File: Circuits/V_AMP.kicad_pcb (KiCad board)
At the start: 2 copper layers, 103 x 153.5 mm, 138 parts, among them P1 INPUT, P2 GAIN_ADJ, P3 OUTPUT (0-5V), P4 POWER, U1 wOPA177, U2 LM393, U3 OPA177

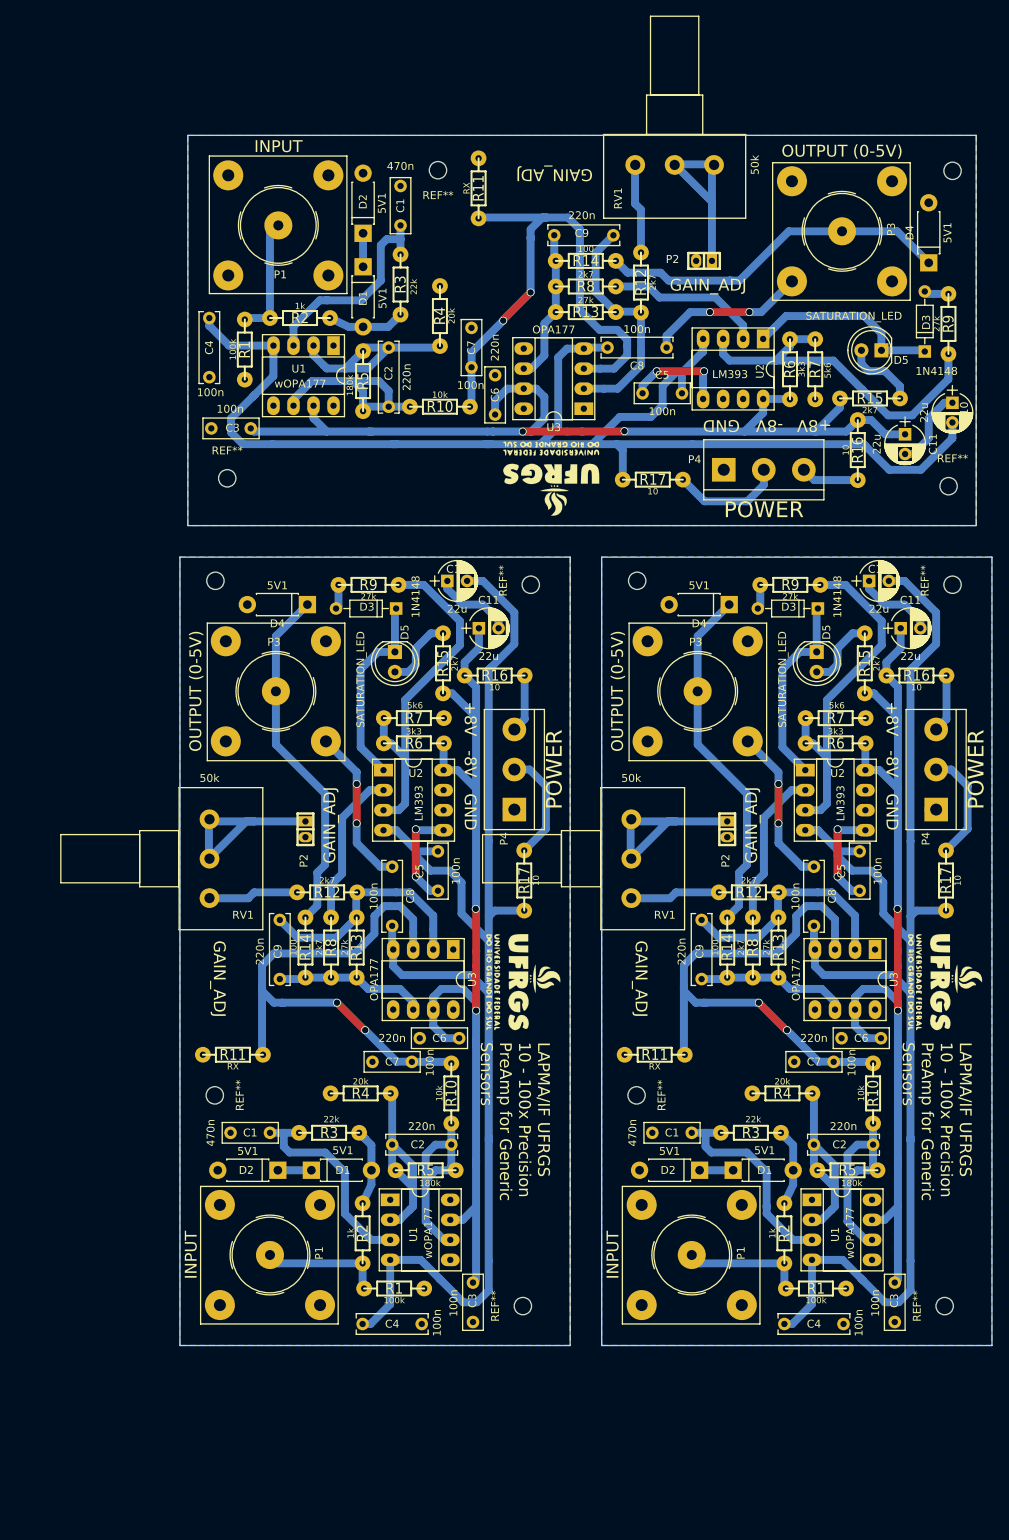
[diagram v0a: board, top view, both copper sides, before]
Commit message: EDIT: Page SETUP
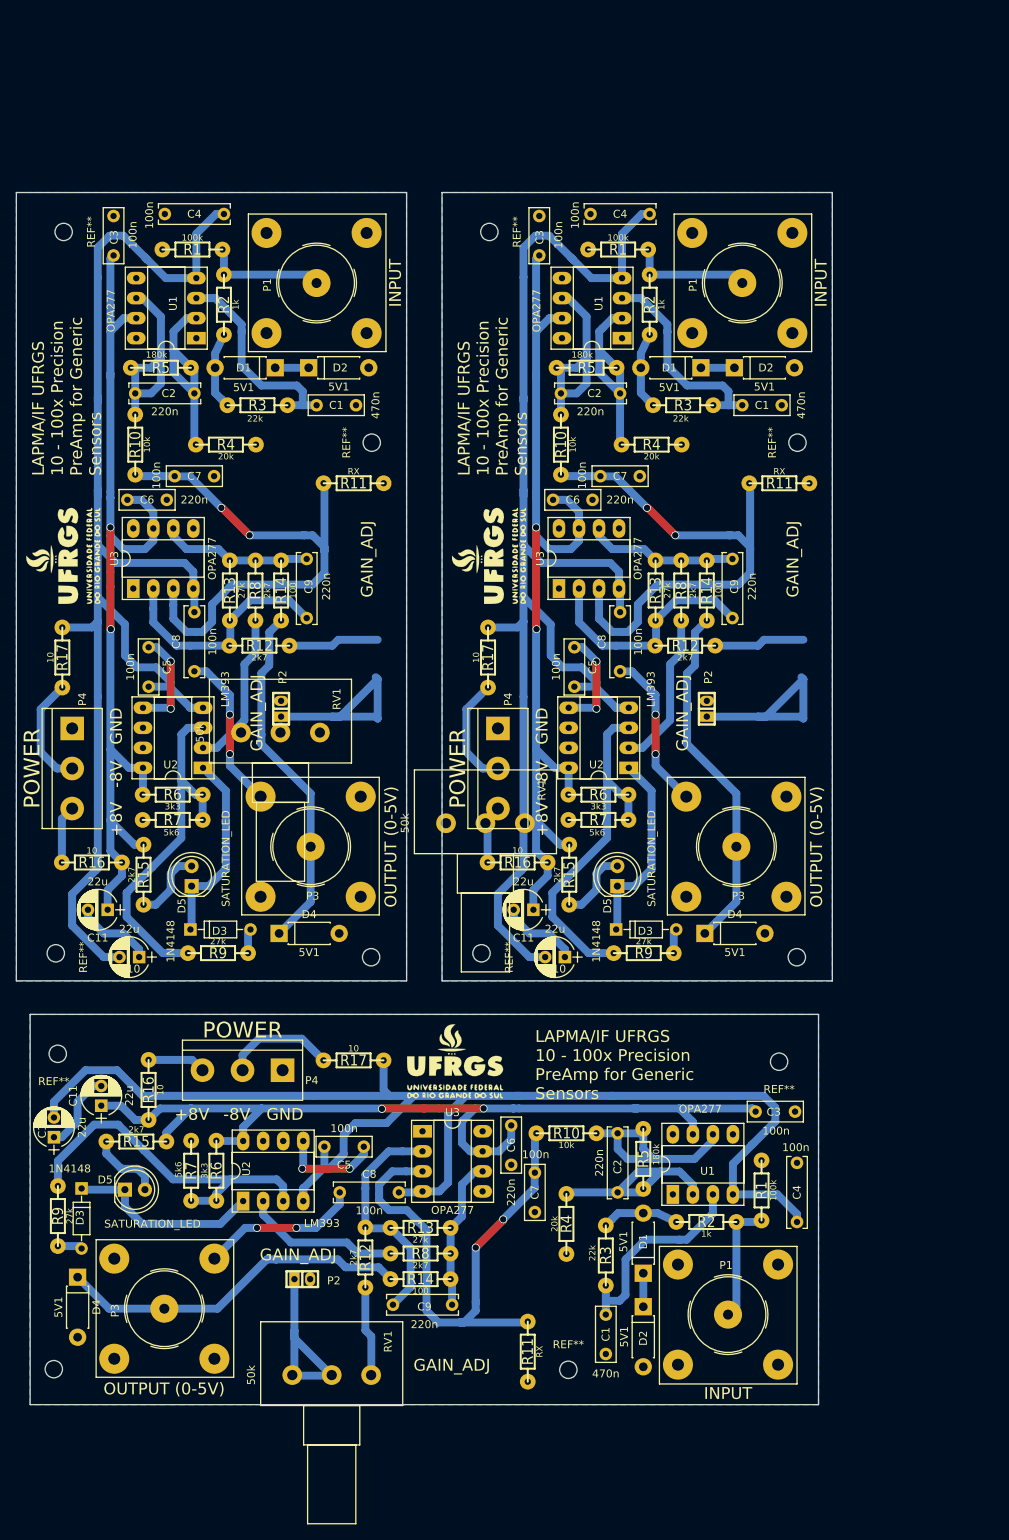
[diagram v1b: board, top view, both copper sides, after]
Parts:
- removed the C1 at (135.9, 152.0)
- removed the C1 at (82.4, 152.0)
- removed the C10 at (158.4, 82.0)
- removed the C10 at (104.9, 82.0)
- removed the C11 at (162.4, 88.0)
- removed the C11 at (108.9, 88.0)
- removed the C2 at (158.9, 153.5)
- removed the C2 at (105.4, 153.5)
- removed the C3 at (161.7, 176.0)
- removed the C3 at (108.2, 176.0)
- removed the C4 at (155.2, 176.3)
- removed the C4 at (101.7, 176.3)
- removed the C5 at (157.2, 121.3)
- removed the C5 at (103.7, 121.3)
- removed the C6 at (154.9, 140.0)
- removed the C6 at (101.4, 140.0)
- removed the C7 at (148.9, 143.0)
- removed the C7 at (95.4, 143.0)
- removed the C8 at (151.4, 118.3)
- removed the C8 at (97.9, 118.3)
- removed the C9 at (137.2, 125.0)
- removed the C9 at (83.7, 125.0)
- removed the D1 at (141.2, 156.8)
- removed the D1 at (87.7, 156.8)
- removed the D2 at (136.9, 156.8)
- removed the D2 at (83.4, 156.8)
- removed the D3 at (151.9, 85.5)
- removed the D3 at (98.4, 85.5)
- removed the D4 at (140.7, 85.0)
- removed the D4 at (87.2, 85.0)
- removed the D5 at (151.8, 91.0)
- removed the D5 at (98.3, 91.0)
- removed the G*** at (168.0, 133.0)
- removed the G*** at (114.5, 133.0)
- removed the P1 at (135.9, 167.5)
- removed the P1 at (82.4, 167.5)
- removed the P2 at (140.4, 113.5)
- removed the P2 at (86.9, 113.5)
- removed the P3 at (136.7, 96.0)
- removed the P3 at (83.2, 96.0)
- removed the P4 at (166.9, 111.0)
- removed the P4 at (113.4, 111.0)
- removed the R1 at (151.7, 171.8)
- removed the R1 at (98.2, 171.8)
- removed the R10 at (158.9, 147.0)
- removed the R10 at (105.4, 147.0)
- removed the R11 at (131.2, 142.1)
- removed the R11 at (77.7, 142.1)
- removed the R12 at (143.2, 121.5)
- removed the R12 at (89.7, 121.5)
- removed the R13 at (146.9, 128.5)
- removed the R13 at (93.4, 128.5)
- removed the R14 at (140.4, 128.5)
- removed the R14 at (86.9, 128.5)
- removed the R15 at (157.9, 92.5)
- removed the R15 at (104.4, 92.5)
- removed the R16 at (164.4, 94.0)
- removed the R16 at (110.9, 94.0)
- removed the R17 at (168.2, 120.0)
- removed the R17 at (114.7, 120.0)
- removed the R2 at (147.7, 164.8)
- removed the R2 at (94.2, 164.8)
- removed the R3 at (143.4, 152.0)
- removed the R3 at (89.9, 152.0)
- removed the R4 at (147.4, 147.0)
- removed the R4 at (93.9, 147.0)
- removed the R5 at (155.7, 156.8)
- removed the R5 at (102.2, 156.8)
- removed the R6 at (154.2, 102.6)
- removed the R6 at (100.7, 102.6)
- removed the R7 at (154.2, 99.4)
- removed the R7 at (100.7, 99.4)
- removed the R8 at (143.7, 128.5)
- removed the R8 at (90.2, 128.5)
- removed the R9 at (148.4, 82.5)
- removed the R9 at (94.9, 82.5)
- removed the REF** at (75.5, 82.0)
- removed the REF** at (75.4, 147.3)
- removed the REF** at (114.5, 174.0)
- removed the REF** at (168.0, 174.0)
- removed the REF** at (128.9, 147.3)
- removed the REF** at (129.0, 82.0)
- removed the REF** at (169.0, 82.5)
- removed the REF** at (115.5, 82.5)
- removed the RV1 at (128.2, 112.2)
- removed the RV1 at (74.8, 112.2)
- removed the U1 at (151.2, 160.5)
- removed the U1 at (97.7, 160.5)
- removed the U2 at (150.3, 106.0)
- removed the U2 at (96.8, 106.0)
- removed the U3 at (159.2, 128.8)
- removed the U3 at (105.7, 128.8)
- added C1: 470n, Capacitors_THT:C_Rect_L7.0mm_W2.5mm_P5.00mm, F.Cu at (142.3, 59.7)
- added C1: 470n, Capacitors_THT:C_Rect_L7.0mm_W2.5mm_P5.00mm, F.Cu at (88.3, 59.7)
- added C10: 22u, Capacitors_THT:CP_Radial_D5.0mm_P2.50mm, F.Cu at (119.8, 129.7)
- added C10: 22u, Capacitors_THT:CP_Radial_D5.0mm_P2.50mm, F.Cu at (65.8, 129.7)
- added C11: 22u, Capacitors_THT:CP_Radial_D5.0mm_P2.50mm, F.Cu at (115.8, 123.7)
- added C11: 22u, Capacitors_THT:CP_Radial_D5.0mm_P2.50mm, F.Cu at (61.8, 123.7)
- added C2: 220n, Capacitors_THT:C_Rect_L9.0mm_W2.5mm_P7.50mm_MKT, F.Cu at (119.3, 58.2)
- added C2: 220n, Capacitors_THT:C_Rect_L9.0mm_W2.5mm_P7.50mm_MKT, F.Cu at (65.3, 58.2)
- added C3: 100n, Capacitors_THT:C_Rect_L7.0mm_W2.5mm_P5.00mm, F.Cu at (116.6, 35.7)
- added C3: 100n, Capacitors_THT:C_Rect_L7.0mm_W2.5mm_P5.00mm, F.Cu at (62.6, 35.7)
- added C4: 100n, Capacitors_THT:C_Rect_L9.0mm_W2.5mm_P7.50mm_MKT, F.Cu at (123.1, 35.5)
- added C4: 100n, Capacitors_THT:C_Rect_L9.0mm_W2.5mm_P7.50mm_MKT, F.Cu at (69.1, 35.5)
- added C5: 100n, Capacitors_THT:C_Rect_L7.0mm_W2.5mm_P5.00mm, F.Cu at (121.0, 90.4)
- added C5: 100n, Capacitors_THT:C_Rect_L7.0mm_W2.5mm_P5.00mm, F.Cu at (67.0, 90.4)
- added C6: 100n, Capacitors_THT:C_Rect_L7.0mm_W2.5mm_P5.00mm, F.Cu at (123.3, 71.7)
- added C6: 100n, Capacitors_THT:C_Rect_L7.0mm_W2.5mm_P5.00mm, F.Cu at (69.3, 71.7)
- added C7: 220n, Capacitors_THT:C_Rect_L7.0mm_W2.5mm_P5.00mm, F.Cu at (129.3, 68.7)
- added C7: 220n, Capacitors_THT:C_Rect_L7.0mm_W2.5mm_P5.00mm, F.Cu at (75.3, 68.7)
- added C8: 100n, Capacitors_THT:C_Rect_L9.0mm_W2.5mm_P7.50mm_MKT, F.Cu at (126.8, 93.5)
- added C8: 100n, Capacitors_THT:C_Rect_L9.0mm_W2.5mm_P7.50mm_MKT, F.Cu at (72.8, 93.5)
- added C9: 220n, Capacitors_THT:C_Rect_L9.0mm_W2.5mm_P7.50mm_MKT, F.Cu at (141.1, 86.7)
- added C9: 220n, Capacitors_THT:C_Rect_L9.0mm_W2.5mm_P7.50mm_MKT, F.Cu at (87.1, 86.7)
- added D1: 5V1, Diodes_THT:D_DO-41_SOD81_P7.62mm_Horizontal, F.Cu at (137.1, 55.0)
- added D1: 5V1, Diodes_THT:D_DO-41_SOD81_P7.62mm_Horizontal, F.Cu at (83.1, 55.0)
- added D2: 5V1, Diodes_THT:D_DO-41_SOD81_P7.62mm_Horizontal, F.Cu at (141.3, 55.0)
- added D2: 5V1, Diodes_THT:D_DO-41_SOD81_P7.62mm_Horizontal, F.Cu at (87.3, 55.0)
- added D3: 1N4148, Diodes_THT:D_DO-35_SOD27_P7.62mm_Horizontal, F.Cu at (126.3, 126.2)
- added D3: 1N4148, Diodes_THT:D_DO-35_SOD27_P7.62mm_Horizontal, F.Cu at (72.3, 126.2)
- added D4: 5V1, Diodes_THT:D_DO-41_SOD81_P7.62mm_Horizontal, F.Cu at (137.6, 126.7)
- added D4: 5V1, Diodes_THT:D_DO-41_SOD81_P7.62mm_Horizontal, F.Cu at (83.6, 126.7)
- added D5: SATURATION_LED, LEDs:LED_D5.0mm, F.Cu at (126.5, 120.7)
- added D5: SATURATION_LED, LEDs:LED_D5.0mm, F.Cu at (72.5, 120.7)
- added G***: LOGO, Symbols:ufrgs, F.Cu at (110.2, 78.8)
- added G***: LOGO, Symbols:ufrgs, F.Cu at (56.2, 78.8)
- added P1: INPUT, Connectors:bnc-ci, F.Cu at (142.3, 44.2)
- added P1: INPUT, Connectors:bnc-ci, F.Cu at (88.3, 44.2)
- added P2: GAIN_ADJ, w_pin_strip:pin_strip_2mm_2, F.Cu at (137.8, 98.2)
- added P2: GAIN_ADJ, w_pin_strip:pin_strip_2mm_2, F.Cu at (83.8, 98.2)
- added P3: OUTPUT (0-5V), Connectors:bnc-ci, F.Cu at (141.6, 115.7)
- added P3: OUTPUT (0-5V), Connectors:bnc-ci, F.Cu at (87.6, 115.7)
- added P4: POWER, Connectors:bornier3, F.Cu at (111.3, 100.7)
- added P4: POWER, Connectors:bornier3, F.Cu at (57.3, 100.7)
- added R1: 100k, w_pth_resistors:RC03, F.Cu at (126.6, 40.0)
- added R1: 100k, w_pth_resistors:RC03, F.Cu at (72.6, 40.0)
- added R10: 10k, w_pth_resistors:RC03, F.Cu at (119.3, 64.7)
- added R10: 10k, w_pth_resistors:RC03, F.Cu at (65.3, 64.7)
- added R11: RX, w_pth_resistors:RC03, F.Cu at (147.0, 69.6)
- added R11: RX, w_pth_resistors:RC03, F.Cu at (93.0, 69.6)
- added R12: 2k7, w_pth_resistors:RC03, F.Cu at (135.1, 90.2)
- added R12: 2k7, w_pth_resistors:RC03, F.Cu at (81.1, 90.2)
- added R13: 27k, w_pth_resistors:RC03, F.Cu at (131.3, 83.2)
- added R13: 27k, w_pth_resistors:RC03, F.Cu at (77.3, 83.2)
- added R14: 100, w_pth_resistors:RC03, F.Cu at (137.8, 83.2)
- added R14: 100, w_pth_resistors:RC03, F.Cu at (83.8, 83.2)
- added R15: 2k7, w_pth_resistors:RC03, F.Cu at (120.4, 119.3)
- added R15: 2k7, w_pth_resistors:RC03, F.Cu at (66.4, 119.3)
- added R16: 10, w_pth_resistors:RC03, F.Cu at (113.8, 117.7)
- added R16: 10, w_pth_resistors:RC03, F.Cu at (59.8, 117.7)
- added R17: 10, w_pth_resistors:RC03, F.Cu at (110.1, 91.7)
- added R17: 10, w_pth_resistors:RC03, F.Cu at (56.1, 91.7)
- added R2: 1k, w_pth_resistors:RC03, F.Cu at (130.6, 47.0)
- added R2: 1k, w_pth_resistors:RC03, F.Cu at (76.6, 47.0)
- added R3: 22k, w_pth_resistors:RC03, F.Cu at (134.8, 59.7)
- added R3: 22k, w_pth_resistors:RC03, F.Cu at (80.8, 59.7)
- added R4: 20k, w_pth_resistors:RC03, F.Cu at (130.8, 64.7)
- added R4: 20k, w_pth_resistors:RC03, F.Cu at (76.8, 64.7)
- added R5: 180k, w_pth_resistors:RC03, F.Cu at (122.6, 55.0)
- added R5: 180k, w_pth_resistors:RC03, F.Cu at (68.6, 55.0)
- added R6: 3k3, w_pth_resistors:RC03, F.Cu at (124.1, 109.1)
- added R6: 3k3, w_pth_resistors:RC03, F.Cu at (70.1, 109.1)
- added R7: 5k6, w_pth_resistors:RC03, F.Cu at (124.1, 112.3)
- added R7: 5k6, w_pth_resistors:RC03, F.Cu at (70.1, 112.3)
- added R8: 2k7, w_pth_resistors:RC03, F.Cu at (134.6, 83.2)
- added R8: 2k7, w_pth_resistors:RC03, F.Cu at (80.6, 83.2)
- added R9: 27k, w_pth_resistors:RC03, F.Cu at (129.8, 129.2)
- added R9: 27k, w_pth_resistors:RC03, F.Cu at (75.8, 129.2)
- added REF**: MountingHole_2.2mm_M2, Mounting_Holes:MountingHole_2.2mm_M2, F.Cu at (110.2, 37.8)
- added REF**: MountingHole_2.2mm_M2, Mounting_Holes:MountingHole_2.2mm_M2, F.Cu at (149.3, 64.5)
- added REF**: MountingHole_2.2mm_M2, Mounting_Holes:MountingHole_2.2mm_M2, F.Cu at (149.2, 129.8)
- added REF**: MountingHole_2.2mm_M2, Mounting_Holes:MountingHole_2.2mm_M2, F.Cu at (109.2, 129.2)
- added REF**: MountingHole_2.2mm_M2, Mounting_Holes:MountingHole_2.2mm_M2, F.Cu at (55.2, 129.2)
- added REF**: MountingHole_2.2mm_M2, Mounting_Holes:MountingHole_2.2mm_M2, F.Cu at (95.2, 129.8)
- added REF**: MountingHole_2.2mm_M2, Mounting_Holes:MountingHole_2.2mm_M2, F.Cu at (95.3, 64.5)
- added REF**: MountingHole_2.2mm_M2, Mounting_Holes:MountingHole_2.2mm_M2, F.Cu at (56.2, 37.8)
- added RV1: 50k, Potentiometers:Potentiometer_Alps_RK163_Single_Vertical, F.Cu at (104.8, 112.8)
- added RV1: 50k, Potentiometers:Potentiometer_Alps_RK163_Single_Vertical, F.Cu at (78.8, 101.2)
- added U1: OPA277, Housings_DIP:DIP-8_W7.62mm_Socket_LongPads, F.Cu at (127.1, 51.2)
- added U1: OPA277, Housings_DIP:DIP-8_W7.62mm_Socket_LongPads, F.Cu at (73.1, 51.2)
- added U2: LM393, Housings_DIP:DIP-8_W7.62mm_Socket_LongPads, F.Cu at (127.9, 105.7)
- added U2: LM393, Housings_DIP:DIP-8_W7.62mm_Socket_LongPads, F.Cu at (73.9, 105.7)
- added U3: OPA277, Housings_DIP:DIP-8_W7.62mm_Socket_LongPads, F.Cu at (119.1, 83.0)
- added U3: OPA277, Housings_DIP:DIP-8_W7.62mm_Socket_LongPads, F.Cu at (65.1, 83.0)
- U1: value wOPA177 -> OPA277
- U3: value OPA177 -> OPA277
- moved REF** 190.0 mm to (55.0, 182.0), turned to 0 degrees
- moved D4 168.0 mm to (58.0, 170.3), turned to 270 degrees
- moved RV1 162.6 mm to (85.2, 182.8), turned to 270 degrees
- moved P3 161.4 mm to (69.0, 174.3), turned to 90 degrees
- moved R9 159.9 mm to (55.5, 162.6), turned to 90 degrees
- moved REF** 153.1 mm to (120.3, 182.1), turned to 0 degrees
- moved D3 150.7 mm to (58.5, 159.1), turned to 270 degrees
- moved P1 149.5 mm to (140.5, 175.1), turned to 0 degrees
- moved R11 147.7 mm to (115.1, 179.8), turned to 90 degrees
- moved C10 147.2 mm to (55.0, 152.6), turned to 90 degrees
- moved D5 143.3 mm to (64.0, 159.2), turned to 0 degrees
- moved D2 140.7 mm to (129.8, 174.1), turned to 270 degrees
- moved C1 140.6 mm to (125.0, 175.1), turned to 270 degrees
- moved P2 138.8 mm to (86.5, 170.6), turned to 0 degrees
- moved C9 138.5 mm to (98.0, 173.8), turned to 0 degrees
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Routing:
- net Net-(P4-Pad3): track 23.5 -> 16.1 mm
- net Net-(P2-Pad1): track 76.3 -> 83.7 mm
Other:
- board size 103 x 153.5 mm -> 103.5 x 153.8 mm
